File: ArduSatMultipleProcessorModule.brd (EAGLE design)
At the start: 95.5 x 90.3 mm, 268 parts, among them IC1 ATMEGA328P, IC10 ATMEGA328P, IC11 ATMEGA328P, IC12 ATMEGA328P, IC13 ATMEGA328P, IC14 ATMEGA328P, IC15 ATMEGA328P, IC16 ATMEGA328P, IC17 ATMEGA328P, IC18 ATMEGA328P, IC2 ATMEGA328P, IC3 ATMEGA328P, IC4 ATMEGA328P, IC5 ATMEGA328P, IC6 ATMEGA328P, IC7 ATMEGA328P, IC8 MCP23S17ML, IC9 ATMEGA328P, P1 N1_ICSP, P10 N0_ICSP, P11 N1_ICSP, P12 N0_ICSP, P13 N1_ICSP, P14 N0_ICSP, P15 N1_ICSP, P16 N0_ICSP, P17 N1_ICSP, P2 N0_ICSP, P3 N0_ICSP, P4 N1_ICSP, P5 N1_ICSP, P6 N0_ICSP, P7 N1_ICSP, P8 N0_ICSP, P9 N1_ICSP, Q1 BSS138 N-MOSFET, Q10 2N7002 N-MOSFET, Q11 BSS138 N-MOSFET, Q12 BSS138 N-MOSFET, Q13 2N7002 N-MOSFET, Q14 2N7002 N-MOSFET, Q15 BSS138 N-MOSFET, Q16 BSS138 N-MOSFET, Q17 BSS138 N-MOSFET, Q18 BSS138 N-MOSFET, Q19 BSS138 N-MOSFET, Q2 BSS138 N-MOSFET, Q20 BSS138 N-MOSFET, Q21 BSS138 N-MOSFET, Q22 BSS138 N-MOSFET, Q23 2N7002 N-MOSFET, Q24 2N7002 N-MOSFET, Q25 2N7002 N-MOSFET, Q26 2N7002 N-MOSFET, Q27 BSS138 N-MOSFET, Q28 BSS138 N-MOSFET, Q29 BSS138 N-MOSFET, Q3 BSS138 N-MOSFET, Q30 BSS138 N-MOSFET, Q31 BSS138 N-MOSFET, Q32 BSS138 N-MOSFET, Q33 BSS138 N-MOSFET, Q34 BSS138 N-MOSFET, Q35 2N7002 N-MOSFET, Q36 2N7002 N-MOSFET, Q37 2N7002 N-MOSFET, Q38 2N7002 N-MOSFET, Q39 BSS138 N-MOSFET, Q4 BSS138 N-MOSFET, Q40 BSS138 N-MOSFET, Q41 BSS138 N-MOSFET, Q42 BSS138 N-MOSFET, Q43 BSS138 N-MOSFET, Q44 BSS138 N-MOSFET, Q45 BSS138 N-MOSFET, Q46 BSS138 N-MOSFET, Q47 2N7002 N-MOSFET, Q48 2N7002 N-MOSFET, Q49 2N7002 N-MOSFET, Q5 BSS138 N-MOSFET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

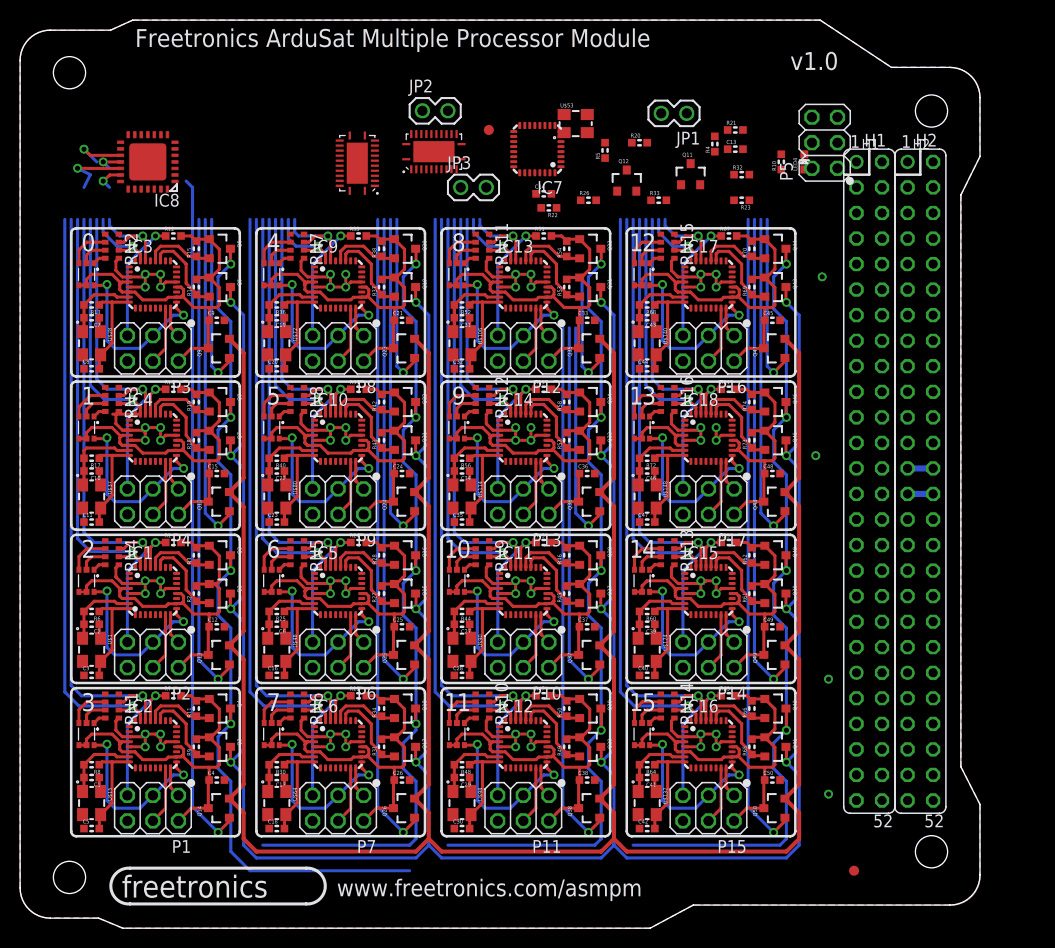
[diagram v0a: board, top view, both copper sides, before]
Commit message: Routing
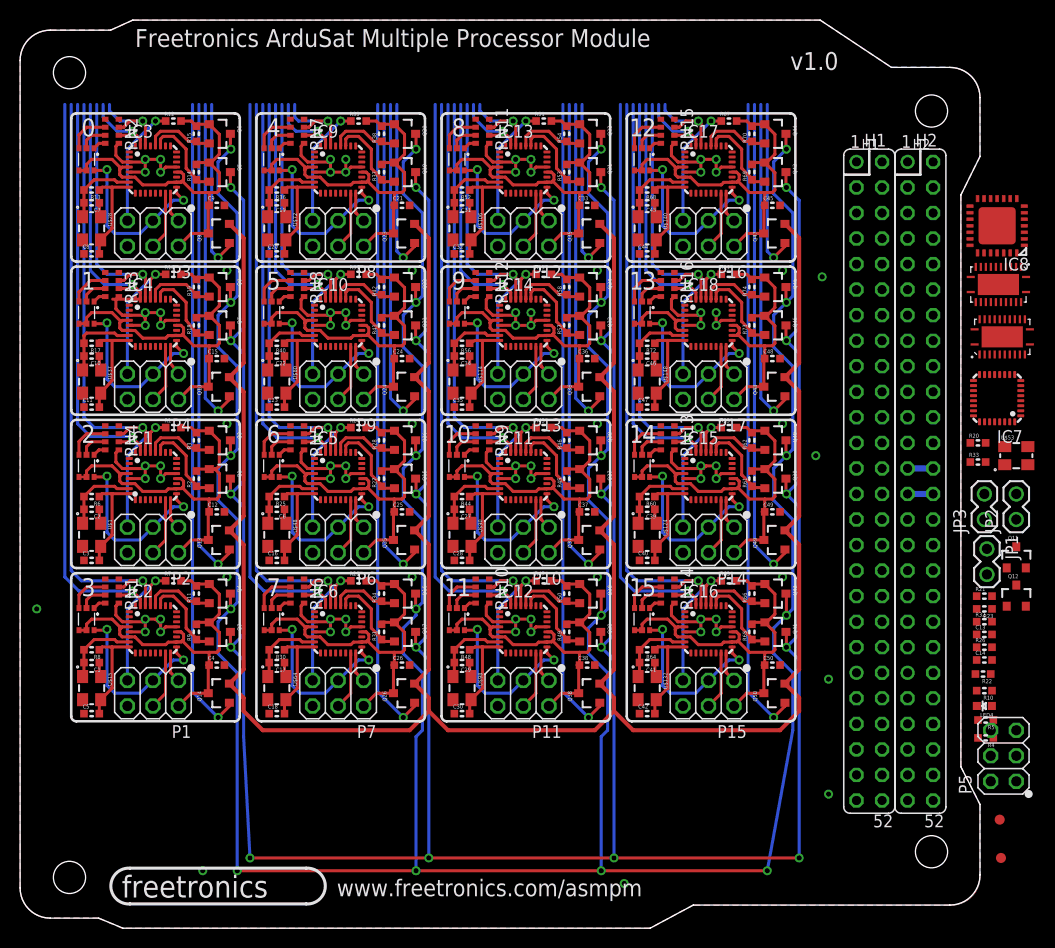
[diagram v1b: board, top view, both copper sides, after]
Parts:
- moved U$21 85.3 mm to (97.4, 10.8)
- moved IC8 84.7 mm to (97.2, 69.8)
- moved JP2 71.7 mm to (99.1, 40.6), turned to 90 degrees
- moved R5 68.1 mm to (96.0, 20.7), turned to 180 degrees
- moved R4 64.9 mm to (96.0, 18.9), turned to 180 degrees
- moved U$60 64.9 mm to (97.3, 64.0), turned to 180 degrees
- moved C14 63.8 mm to (95.9, 26.7)
- moved P5 63.5 mm to (97.8, 17.1)
- moved R22 63.4 mm to (95.8, 25.3)
- moved JP3 61.7 mm to (95.9, 40.6), turned to 90 degrees
- moved U$59 59.4 mm to (97.7, 58.8)
- moved R26 59.4 mm to (95.9, 27.9)
- moved LED4 57.0 mm to (95.9, 22.1), turned to 90 degrees
- moved Q12 56.6 mm to (99.1, 33.0)
- moved R10 56.3 mm to (95.9, 23.6), turned to 180 degrees
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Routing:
- net NODE_SCL: track 337.8 -> 390.7 mm, vias 16 -> 20
- net NODE_SDA: track 313.8 -> 360.8 mm, vias 16 -> 20
- net N11_PWR: track 53.1 -> 63.9 mm
- net N10_PWR: track 37.6 -> 48.4 mm
- net N9_PWR: track 22.1 -> 32.9 mm
- net N2_PWR: track 55.6 -> 48.4 mm, vias 2 -> 1
- net N3_PWR: track 70.9 -> 63.9 mm, vias 2 -> 1
- net N8_PWR: track 11.7 -> 17.4 mm
- net N0_PWR: track 23.1 -> 17.4 mm, vias 2 -> 1
- net +5V_SYS: track 276.2 -> 272.7 mm
- net N1_PWR: track 35.6 -> 32.9 mm, vias 2 -> 1
- net N9_5V: track 38.5 -> 39.7 mm
- net GND: vias 68 -> 83

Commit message: Moved nodes back down to lower part of module
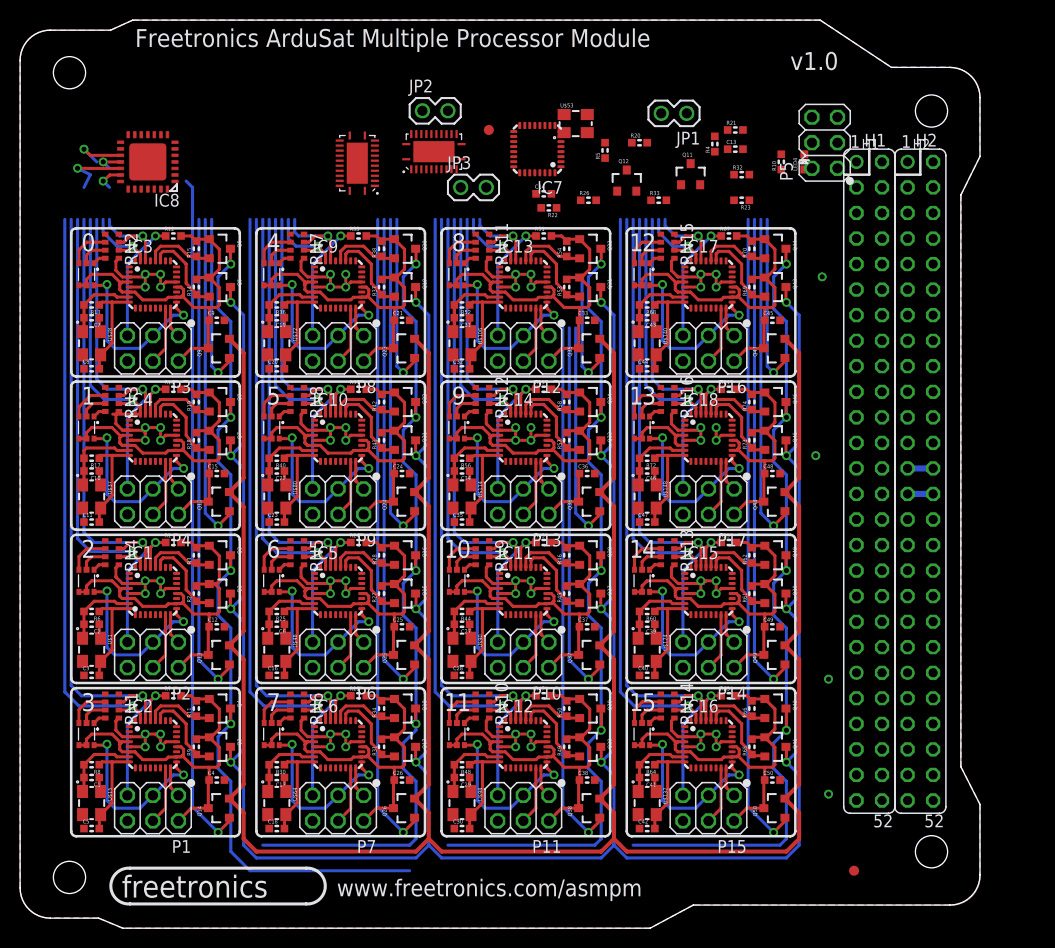
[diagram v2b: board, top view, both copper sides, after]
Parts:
- moved U$21 85.3 mm to (46.6, 79.4)
- moved IC8 84.7 mm to (12.7, 76.2)
- moved JP2 71.7 mm to (40.0, 81.3), turned to 0 degrees
- moved R5 68.1 mm to (58.2, 77.3), turned to 90 degrees
- moved R4 64.9 mm to (69.1, 78.0), turned to 90 degrees
- moved U$60 64.9 mm to (33.5, 76.1), turned to 90 degrees
- moved C14 63.8 mm to (52.1, 73.0)
- moved P5 63.5 mm to (80.0, 78.1)
- moved R22 63.4 mm to (52.6, 71.6)
- moved JP3 61.7 mm to (43.8, 73.7), turned to 0 degrees
- moved U$59 59.4 mm to (41.1, 77.2)
- moved R26 59.4 mm to (56.5, 72.4)
- moved LED4 57.0 mm to (78.0, 76.2), turned to 0 degrees
- moved Q12 56.6 mm to (60.3, 74.3)
- moved R10 56.3 mm to (75.7, 76.2), turned to 90 degrees
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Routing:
- net NODE_SCL: track 390.7 -> 337.8 mm, vias 20 -> 16
- net NODE_SDA: track 360.8 -> 313.8 mm, vias 20 -> 16
- net N11_PWR: track 63.9 -> 53.1 mm
- net N10_PWR: track 48.4 -> 37.6 mm
- net N9_PWR: track 32.9 -> 22.1 mm
- net N2_PWR: track 48.4 -> 55.6 mm, vias 1 -> 2
- net N3_PWR: track 63.9 -> 70.9 mm, vias 1 -> 2
- net N8_PWR: track 17.4 -> 11.7 mm
- net N0_PWR: track 17.4 -> 23.1 mm, vias 1 -> 2
- net +5V_SYS: track 272.7 -> 276.2 mm
- net N1_PWR: track 32.9 -> 35.6 mm, vias 1 -> 2
- net N9_5V: track 39.7 -> 38.5 mm
- net GND: vias 83 -> 68
